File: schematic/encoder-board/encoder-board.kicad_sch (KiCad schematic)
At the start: 61 parts, among them J1 Screw_Terminal_01x02, J10 Screw_Terminal_01x02, J11 Screw_Terminal_01x02, J12 Screw_Terminal_01x02, J13 Screw_Terminal_01x02, J14 Screw_Terminal_01x02, J15 Screw_Terminal_01x02, J16 Screw_Terminal_01x06, J17 Screw_Terminal_01x02, J18 Screw_Terminal_01x02, J19 Screw_Terminal_01x02, J2 Screw_Terminal_01x02, J20 Screw_Terminal_01x02, J21 Screw_Terminal_01x02, J22 Screw_Terminal_01x02, J23 Screw_Terminal_01x02, J24 Screw_Terminal_01x02, J25 Screw_Terminal_01x02, J3 Screw_Terminal_01x02, J4 Screw_Terminal_01x02, J5 Screw_Terminal_01x02, J6 Screw_Terminal_01x02, J7 Screw_Terminal_01x02, J8 Screw_Terminal_01x02, J9 Screw_Terminal_01x02, Q1 2N7002, Q2 2N7002, Q3 2N7002, Q4 2N7002, Q5 2N7002, Q6 2N7002, Q7 2N7002, Q8 2N7002, U1 MCP23017_SO

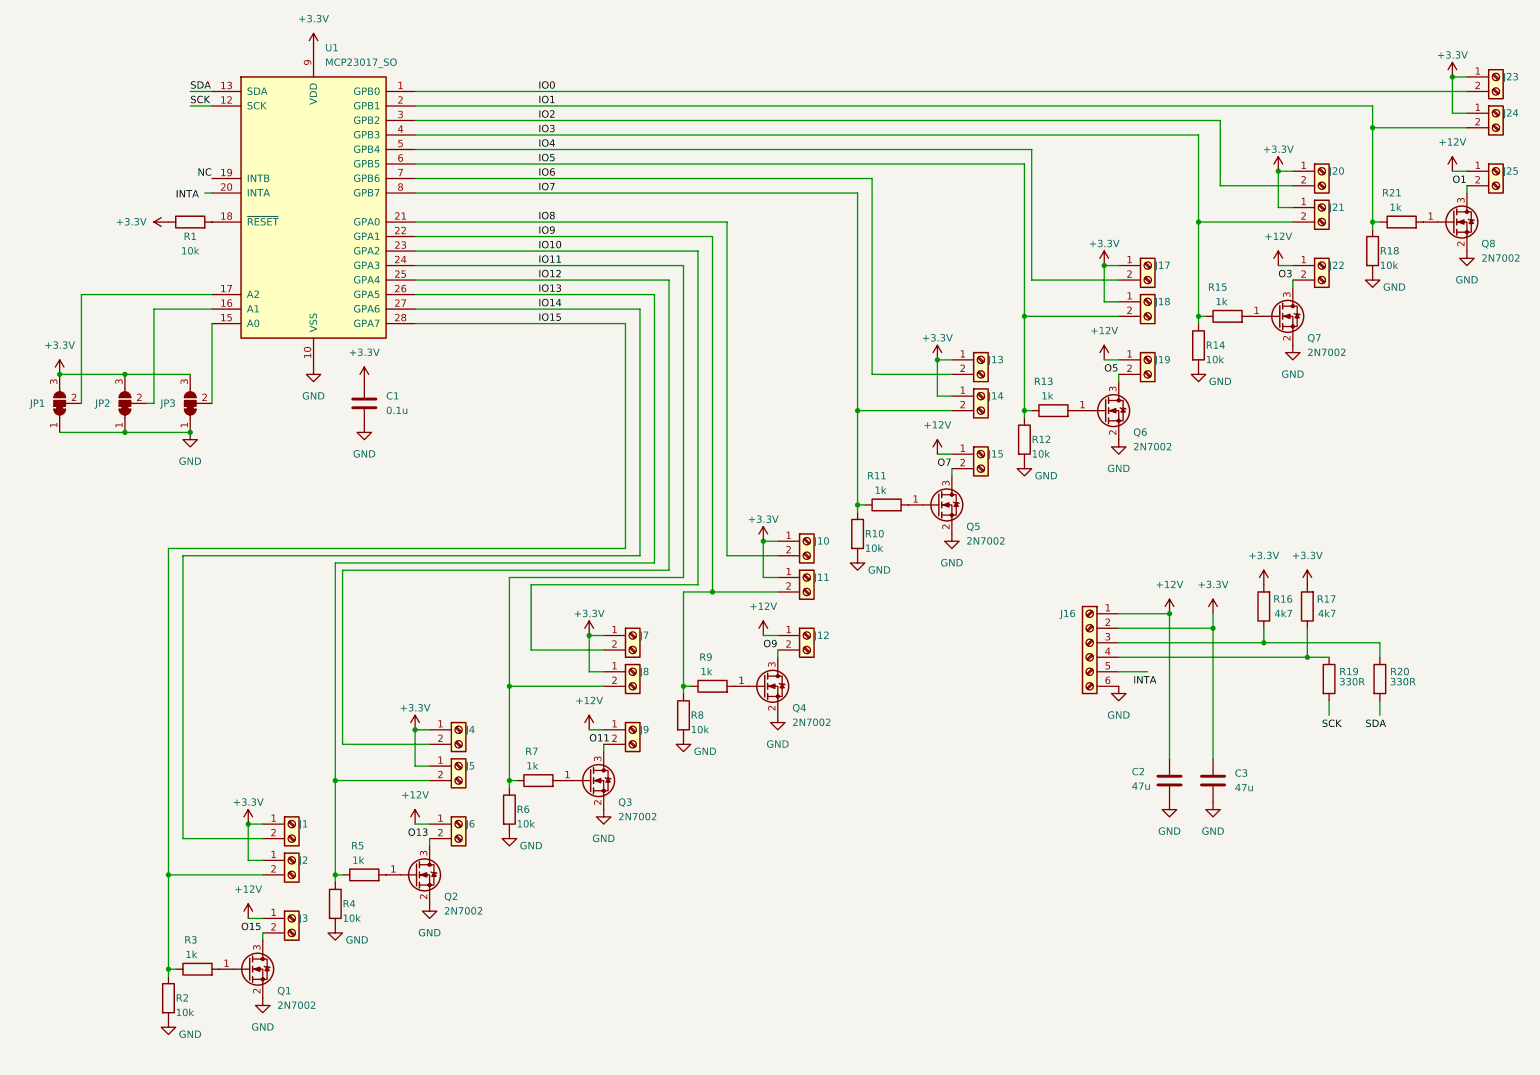
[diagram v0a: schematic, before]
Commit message: schematic updates
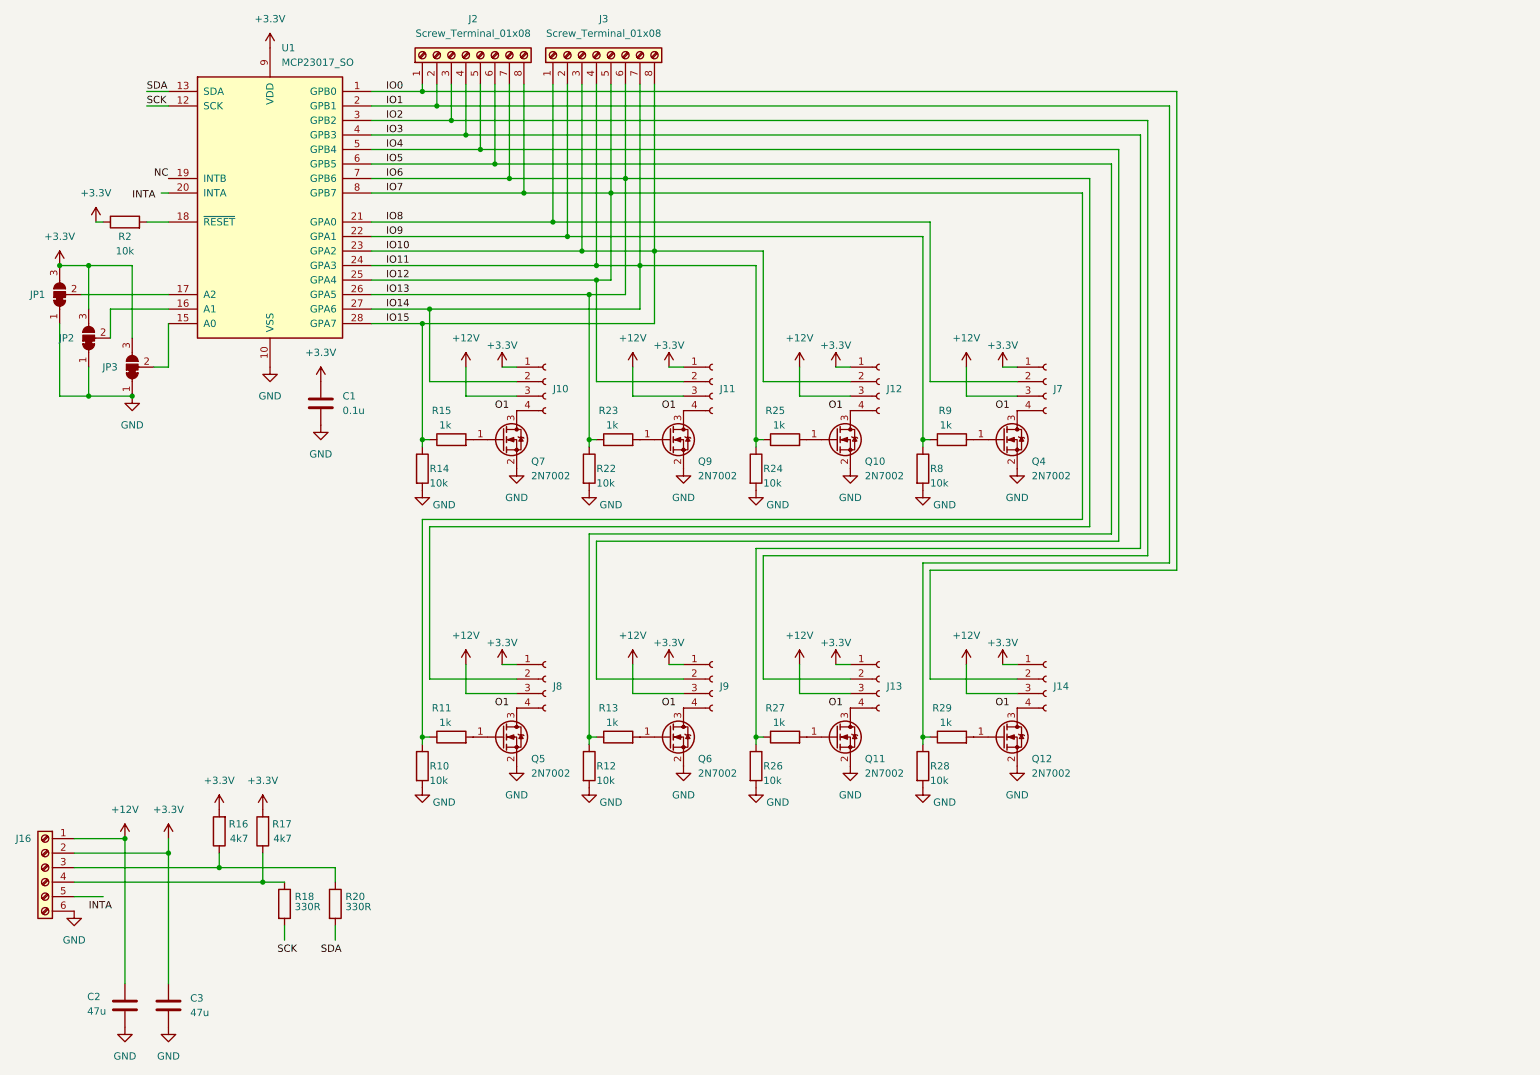
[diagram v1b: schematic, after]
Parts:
- removed J1, J10, J11, J12, J13, J14, J15, J17, J18, J19, J2, J20, J21, J22, J23, J24, J25, J3, J4, J5, J6, J7, J8, J9: Screw_Terminal_01x02, symbol Connector:Screw_Terminal_01x02
- removed Q1, Q2, Q3, Q8: 2N7002, Package_TO_SOT_SMD:SOT-23, symbol Transistor_FET:2N7002
- removed R18, R2, R4, R6: 10k, Resistor_SMD:R_0805_2012Metric, symbol Device:R
- removed R21, R3, R5, R7: 1k, Resistor_SMD:R_0805_2012Metric, symbol Device:R
- added J10, J11, J12, J13, J14, J7, J8, J9: Conn_01x04_Socket, Connector_JST:JST_XH_B4B-XH-AM_1x04_P2.50mm_Vertical, symbol Connector:Conn_01x04_Socket
- added J2, J3: Screw_Terminal_01x08, TerminalBlock:TerminalBlock_bornier-8_P5.08mm, symbol Connector:Screw_Terminal_01x08
- added Q10, Q11, Q12, Q9: 2N7002, Package_TO_SOT_SMD:SOT-23, symbol Transistor_FET:2N7002
- added R22, R24, R26, R28: 10k, Resistor_SMD:R_0805_2012Metric, symbol Device:R
- added R23, R25, R27, R29: 1k, Resistor_SMD:R_0805_2012Metric, symbol Device:R
- C1: footprint (none) -> Capacitor_SMD:C_0805_2012Metric
- C2, C3: footprint (none) -> Capacitor_THT:C_Radial_D6.3mm_H11.0mm_P2.50mm
- J16: footprint (none) -> TerminalBlock:TerminalBlock_bornier-6_P5.08mm
- renumbered R19 to R18, R1 to R2
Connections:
- net IO14 is gone; now on net IO11: U1.27 (GPA6)
- net IO15 is gone; now on net IO10: U1.28 (GPA7)
- net IO6 is gone; now on net IO13: U1.7 (GPB6)
- net IO7 is gone; now on net IO12: R10.1, R11.1, U1.8 (GPB7)
- net +12V: now also J10.3 (Pin_3), J11.3 (Pin_3), J12.3 (Pin_3), J13.3 (Pin_3), J14.3 (Pin_3), J7.3 (Pin_3), J8.3 (Pin_3), J9.3 (Pin_3)
- net +3.3V: now also J10.1 (Pin_1), J11.1 (Pin_1), J12.1 (Pin_1), J13.1 (Pin_1), J14.1 (Pin_1), J7.1 (Pin_1), J8.1 (Pin_1), J9.1 (Pin_1)
- net GND: now also Q10.2 (S), Q11.2 (S), Q12.2 (S), Q9.2 (S), R22.2, R24.2, R26.2, R28.2
- net IO0: now also J14.2 (Pin_2), J2.1 (Pin_1)
- net IO1: now also J2.2 (Pin_2), R28.1, R29.1
- net IO10: now also R14.1, R15.1, J12.2 (Pin_2), J3.3 (Pin_3), J3.8 (Pin_8)
- net IO11: now also J10.2 (Pin_2), J3.4 (Pin_4), J3.7 (Pin_7), R24.1, R25.1
- net IO12: now also J11.2 (Pin_2), J2.8 (Pin_8), J3.5 (Pin_5)
- net IO13: now also J2.7 (Pin_7), J3.6 (Pin_6), J8.2 (Pin_2), R22.1, R23.1
- net IO2: now also J13.2 (Pin_2), J2.3 (Pin_3)
- net IO3: now also J2.4 (Pin_4), R26.1, R27.1; no longer R14.1, R15.1
- net IO4: now also J2.5 (Pin_5), J9.2 (Pin_2)
- net IO5: now also J2.6 (Pin_6)
- net IO8: now also J3.1 (Pin_1), J7.2 (Pin_2)
- net IO9: now also J3.2 (Pin_2)
- net at Q4.3 (D): now also J7.4 (Pin_4)
- net at Q6.3 (D): now also J9.4 (Pin_4)
- net at Q5.3 (D): now also J8.4 (Pin_4)
- net at Q7.3 (D): now also J10.4 (Pin_4)
- new net: Q10.1 (G), R25.2
- new net: J12.4 (Pin_4), Q10.3 (D)
- new net: Q12.1 (G), R29.2
- new net: J11.4 (Pin_4), Q9.3 (D)
- new net: Q11.1 (G), R27.2
- new net: J14.4 (Pin_4), Q12.3 (D)
- new net: Q9.1 (G), R23.2
- new net: J13.4 (Pin_4), Q11.3 (D)
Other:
- moved on the sheet: C1, C2, C3, J16, JP1, JP2, JP3, R16, R17, R18, R2, R20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
